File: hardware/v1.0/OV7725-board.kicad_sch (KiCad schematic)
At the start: 25 parts, among them J11 Conn_01x04, J12 Conn_01x34, J13 Conn_02x10_Odd_Even, U11 TLV62585, U12 CH32V003JxMx, Y2 TFOM24M4RHKCNT2T

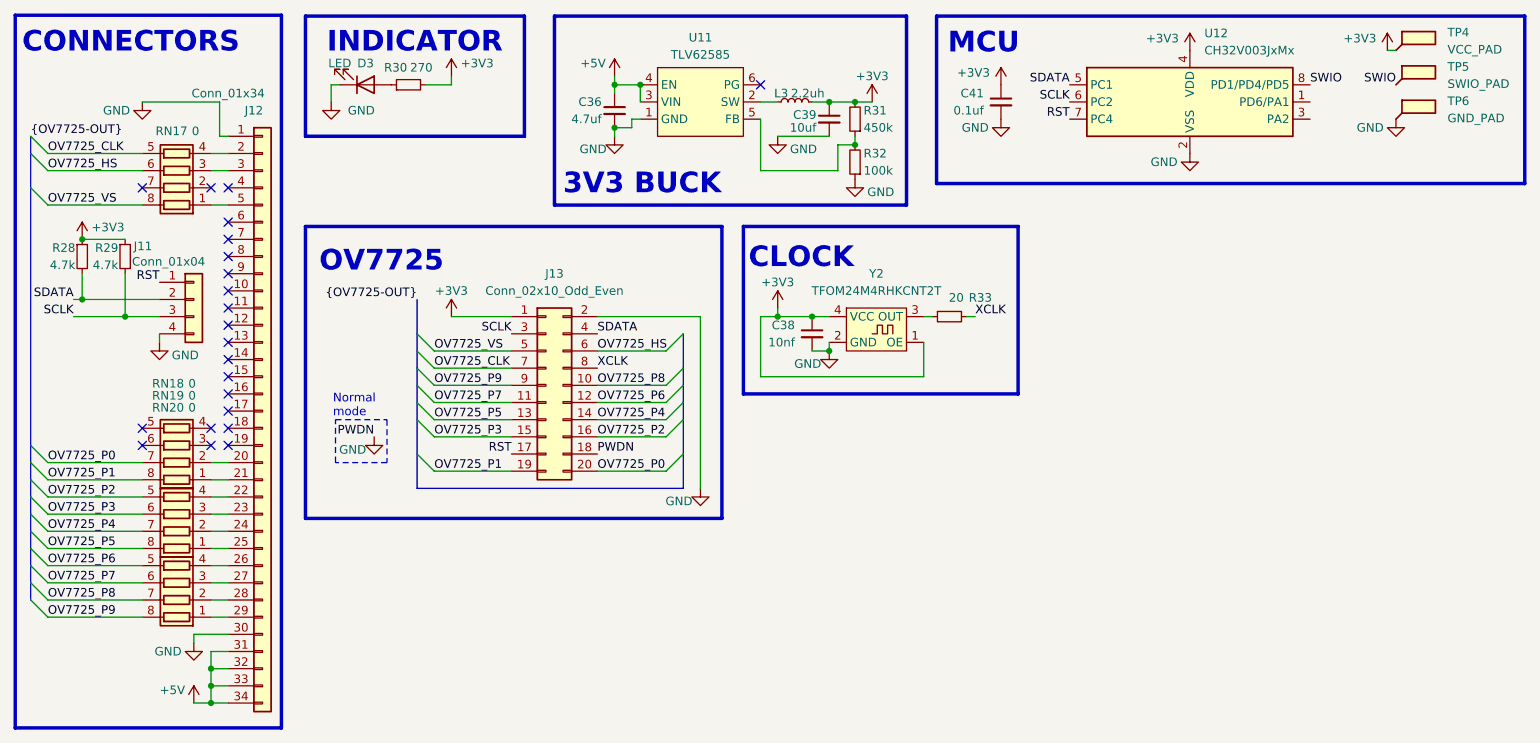
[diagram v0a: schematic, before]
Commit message: first schematic iteration done
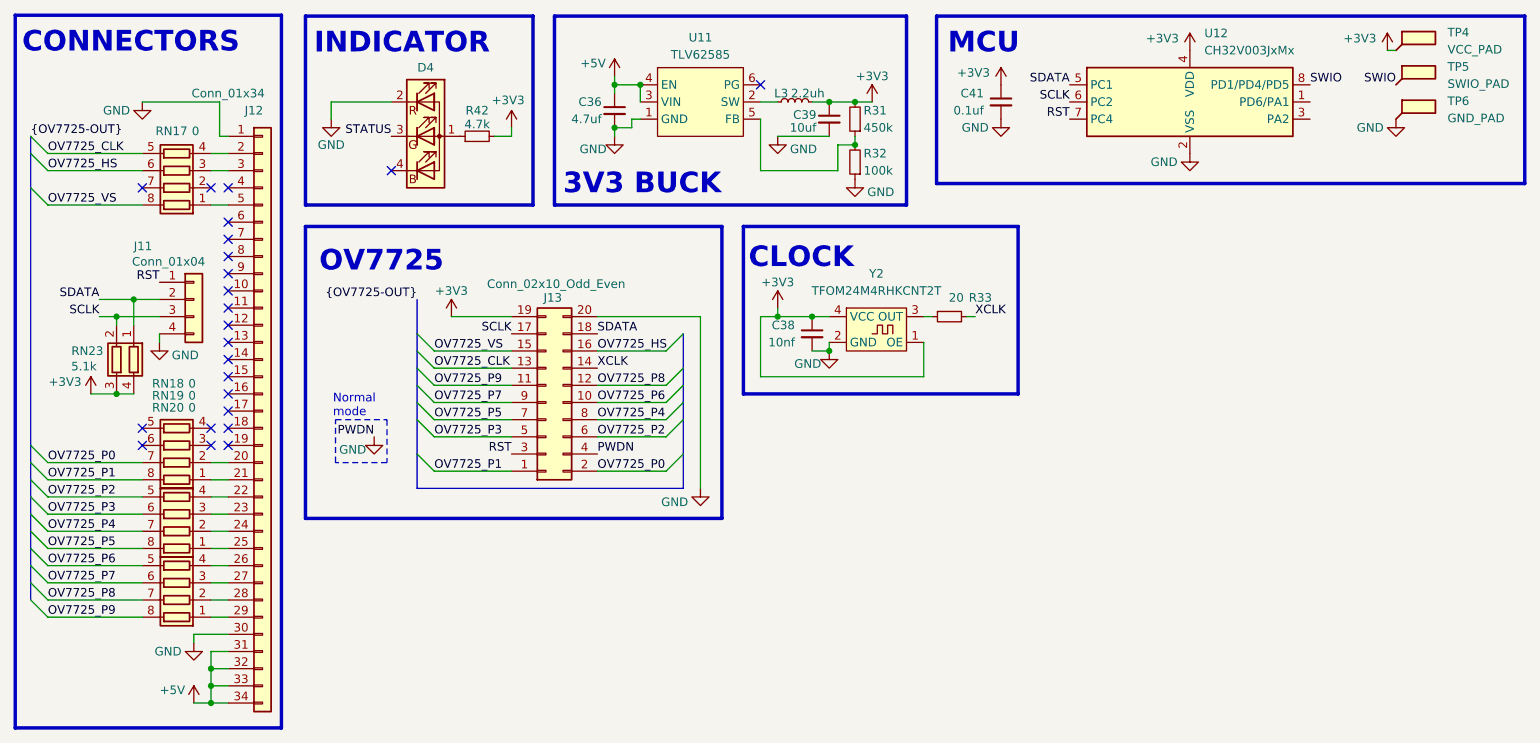
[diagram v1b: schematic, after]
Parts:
- removed D3: LED, LED_SMD:LED_0805_2012Metric, symbol Device:LED
- removed R28, R29: 4.7k, Resistor_SMD:R_0603_1608Metric, symbol Device:R_Small
- removed R30: 270, Resistor_SMD:R_0603_1608Metric, symbol Device:R_Small
- added D4: ~, C779813:LED-SMD_4P-L1.6-W1.5-BR_TZ-P4-1615, symbol Device:LED_ARGB
- added R42: 4.7k, Resistor_SMD:R_0603_1608Metric, symbol Device:R_Small
- added RN23: 5.1k, symbol Device:R_Pack02
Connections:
- net +3V3: now also J13.19 (Pin_19), R42.2, RN23.3 (R2.2), RN23.4 (R1.2); no longer J13.1 (Pin_1)
- net GND: now also J13.20 (Pin_20), J13.4 (Pin_4), D4.2 (RK); no longer J13.18 (Pin_18), J13.2 (Pin_2)
- net OV7725_CLK: now also J13.13 (Pin_13); no longer J13.7 (Pin_7)
- net OV7725_HS: now also J13.16 (Pin_16); no longer J13.6 (Pin_6)
- net OV7725_P0: now also J13.2 (Pin_2); no longer J13.20 (Pin_20)
- net OV7725_P1: now also J13.1 (Pin_1); no longer J13.19 (Pin_19)
- net OV7725_P2: now also J13.6 (Pin_6); no longer J13.16 (Pin_16)
- net OV7725_P3: now also J13.5 (Pin_5); no longer J13.15 (Pin_15)
- net OV7725_P4: now also J13.8 (Pin_8); no longer J13.14 (Pin_14)
- net OV7725_P5: now also J13.7 (Pin_7); no longer J13.13 (Pin_13)
- net OV7725_P6: now also J13.10 (Pin_10); no longer J13.12 (Pin_12)
- net OV7725_P7: now also J13.9 (Pin_9); no longer J13.11 (Pin_11)
- net OV7725_P8: now also J13.12 (Pin_12); no longer J13.10 (Pin_10)
- net OV7725_P9: now also J13.11 (Pin_11); no longer J13.9 (Pin_9)
- net OV7725_VS: now also J13.15 (Pin_15); no longer J13.5 (Pin_5)
- net RST: now also J13.3 (Pin_3); no longer J13.17 (Pin_17)
- net SCLK: now also J13.17 (Pin_17), RN23.2 (R2.1); no longer J13.3 (Pin_3)
- net SDATA: now also J13.18 (Pin_18), RN23.1 (R1.1); no longer J13.4 (Pin_4)
- net XCLK: now also J13.14 (Pin_14); no longer J13.8 (Pin_8)
- new net: D4.1 (A), R42.1
- new net STATUS: D4.3 (GK)
- no-connect marks 22 -> 23
